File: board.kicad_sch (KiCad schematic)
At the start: 6 parts, among them U1 MC68060RC50, U2 XC95144XL-5TQG100C, U3 SST39VF1601C-70-4C-EKE, U4 IS61WV51216BLL-10TLI, U5 IS61WV51216BLL-10TLI, U6 SST39VF1601C-70-4C-EKE

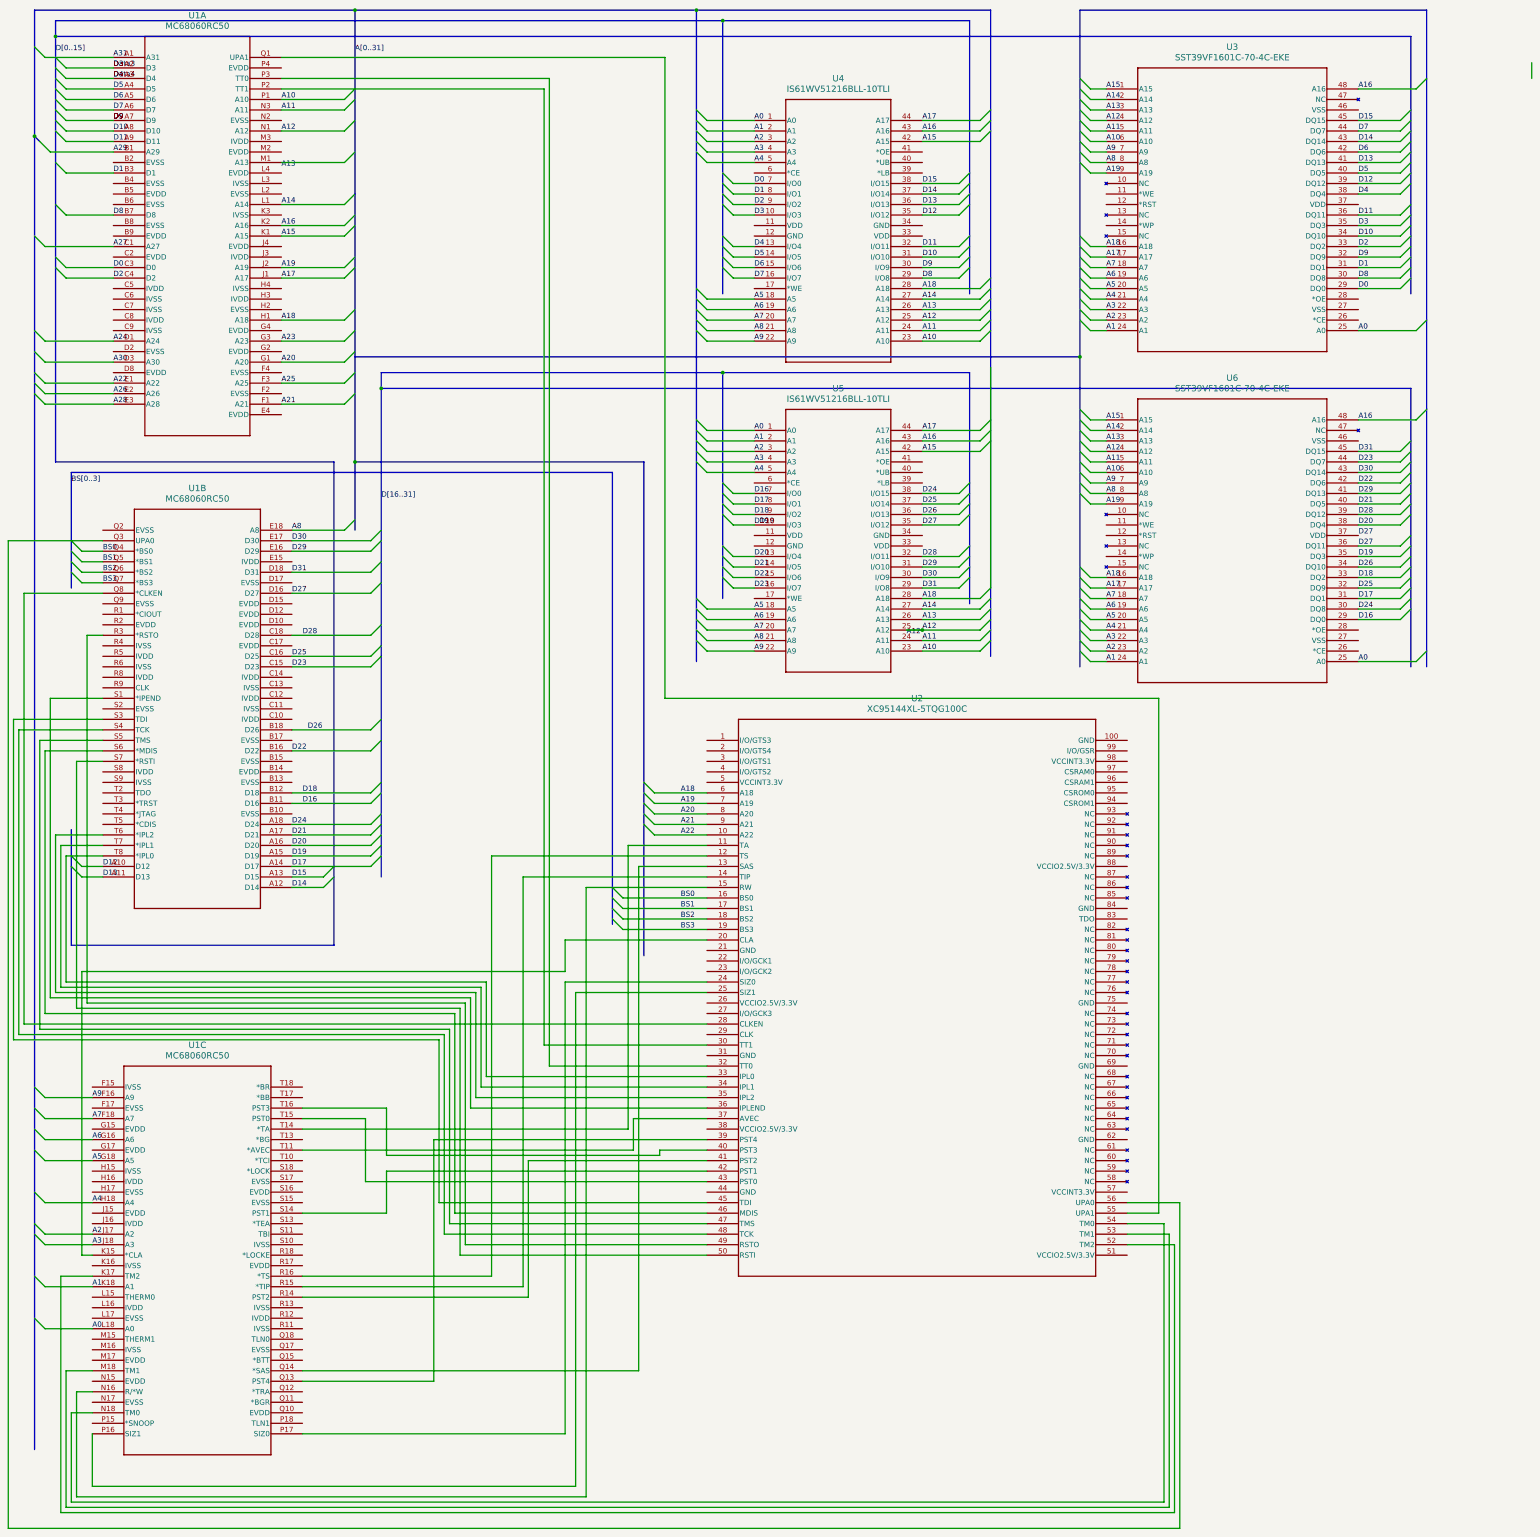
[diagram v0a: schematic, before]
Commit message: First version
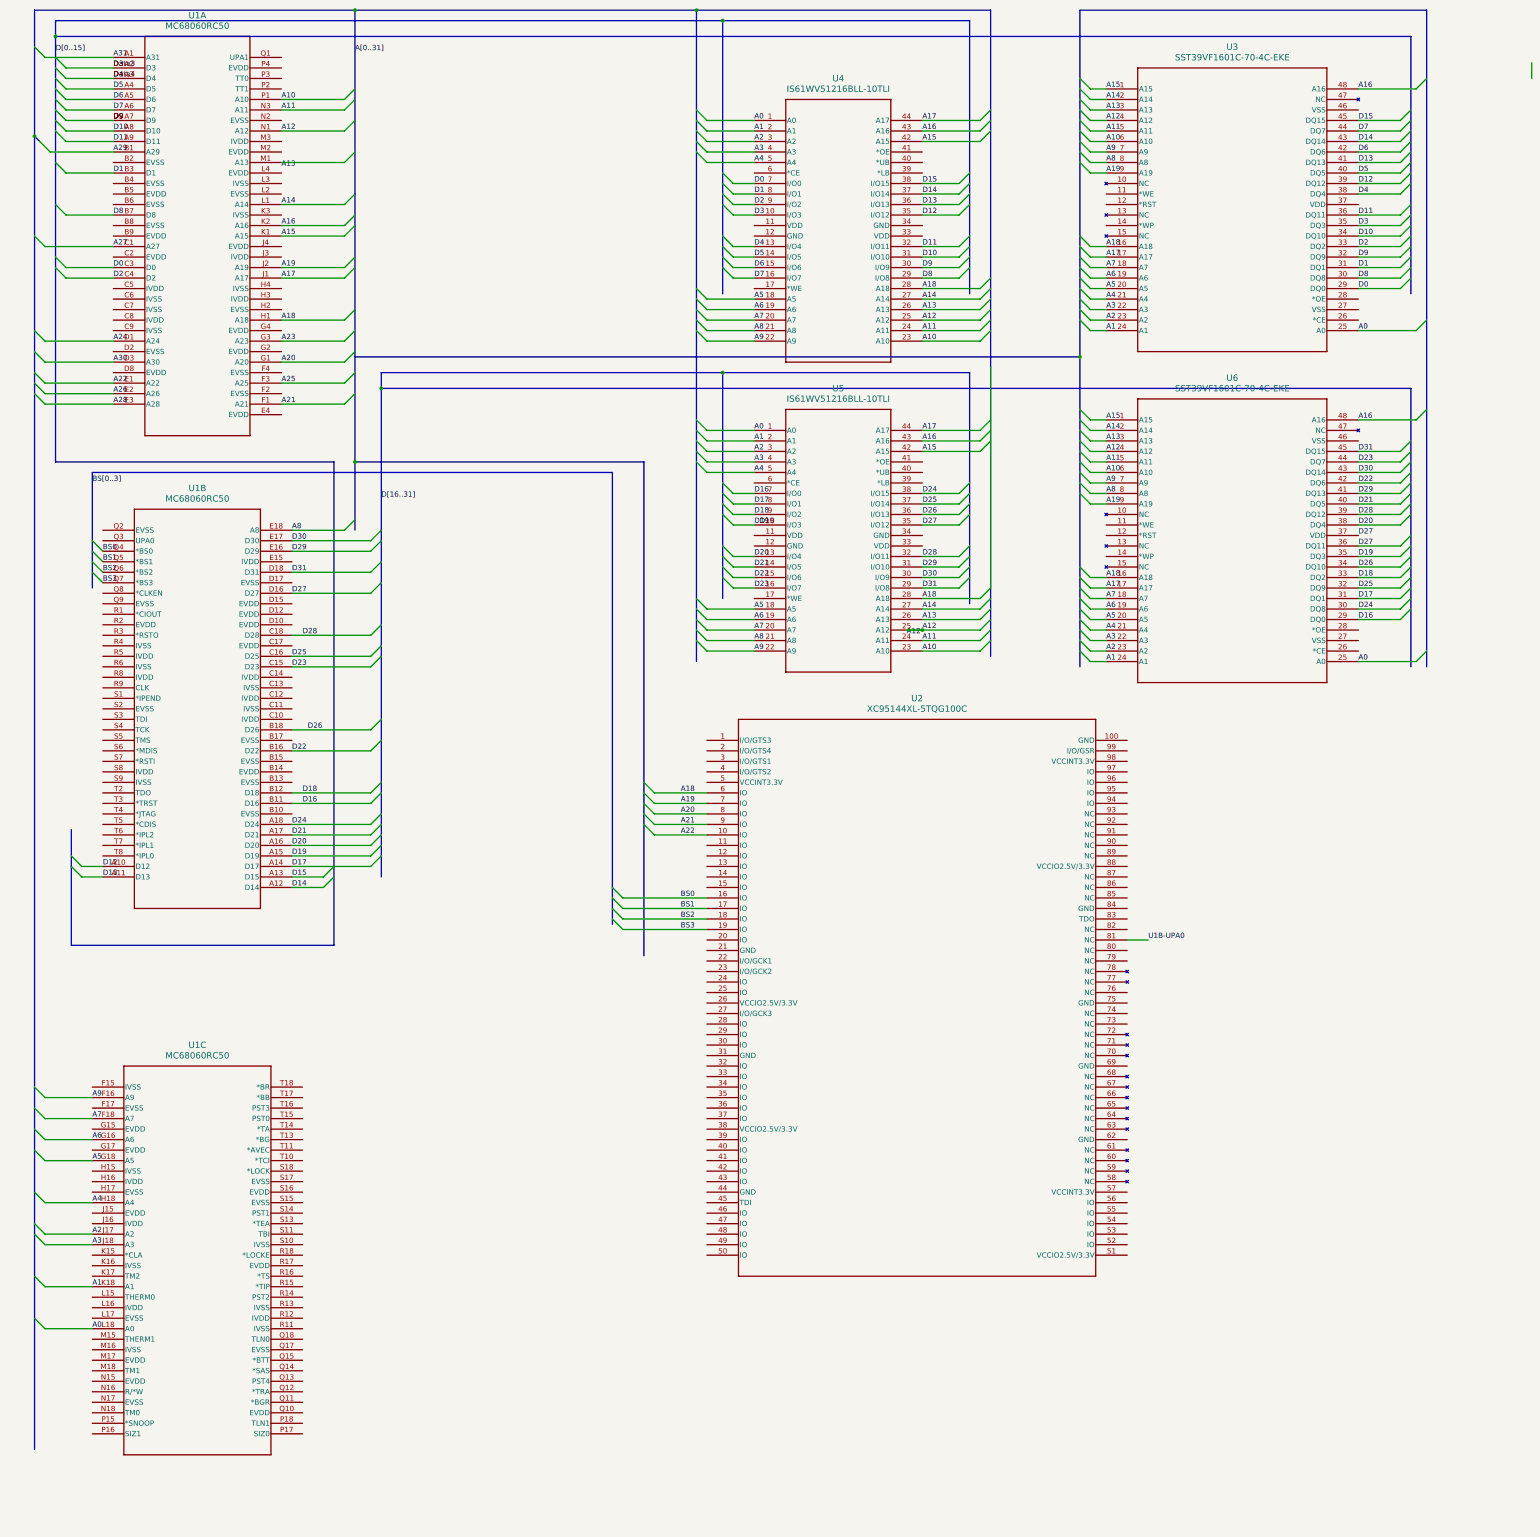
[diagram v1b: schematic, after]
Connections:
- net at U2.11 (IO): no longer U1.T14 (*TA)
- net at U2.12 (IO): no longer U1.R16 (*TS)
- net at U2.13 (IO): no longer U1.Q14 (*SAS)
- net at U2.14 (IO): no longer U1.R15 (*TIP)
- net at U2.15 (IO): no longer U1.N16 (R/*W)
- net at U2.20 (IO): no longer U1.K15 (*CLA)
- net at U2.24 (IO): no longer U1.P17 (SIZ0)
- net at U2.25 (IO): no longer U1.P16 (SIZ1)
- net at U2.28 (IO): no longer U1.Q8 (*CLKEN)
- net at U2.30 (IO): no longer U1.P2 (TT1)
- net at U2.32 (IO): no longer U1.P3 (TT0)
- net at U2.33 (IO): no longer U1.T8 (*IPL0)
- net at U2.34 (IO): no longer U1.T7 (*IPL1)
- net at U2.35 (IO): no longer U1.T6 (*IPL2)
- net at U2.36 (IO): no longer U1.S1 (*IPEND)
- net at U2.37 (IO): no longer U1.T11 (*AVEC)
- net at U2.39 (IO): no longer U1.Q13 (PST4)
- net at U2.40 (IO): no longer U1.T16 (PST3)
- net at U2.41 (IO): no longer U1.R14 (PST2)
- net at U2.42 (IO): no longer U1.S14 (PST1)
- net at U2.43 (IO): no longer U1.T15 (PST0)
- net at U2.45 (TDI): no longer U1.S3 (TDI)
- net at U2.46 (IO): no longer U1.S6 (*MDIS)
- net at U2.47 (IO): no longer U1.S5 (TMS)
- net at U2.48 (IO): no longer U1.S4 (TCK)
- net at U2.49 (IO): no longer U1.R3 (*RSTO)
- net at U2.50 (IO): no longer U1.S7 (*RSTI)
- net at U2.52 (IO): no longer U1.K17 (TM2)
- net at U2.53 (IO): no longer U1.M18 (TM1)
- net at U2.54 (IO): no longer U1.N18 (TM0)
- net at U2.55 (IO): no longer U1.Q1 (UPA1)
- net at U2.56 (IO): no longer U1.Q3 (UPA0)
- net U1B-UPA0: now reaches U2.81 (NC)
